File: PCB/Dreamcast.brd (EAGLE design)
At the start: 73 x 29 mm, 19 parts, among them U1 ESP32DEVKITC

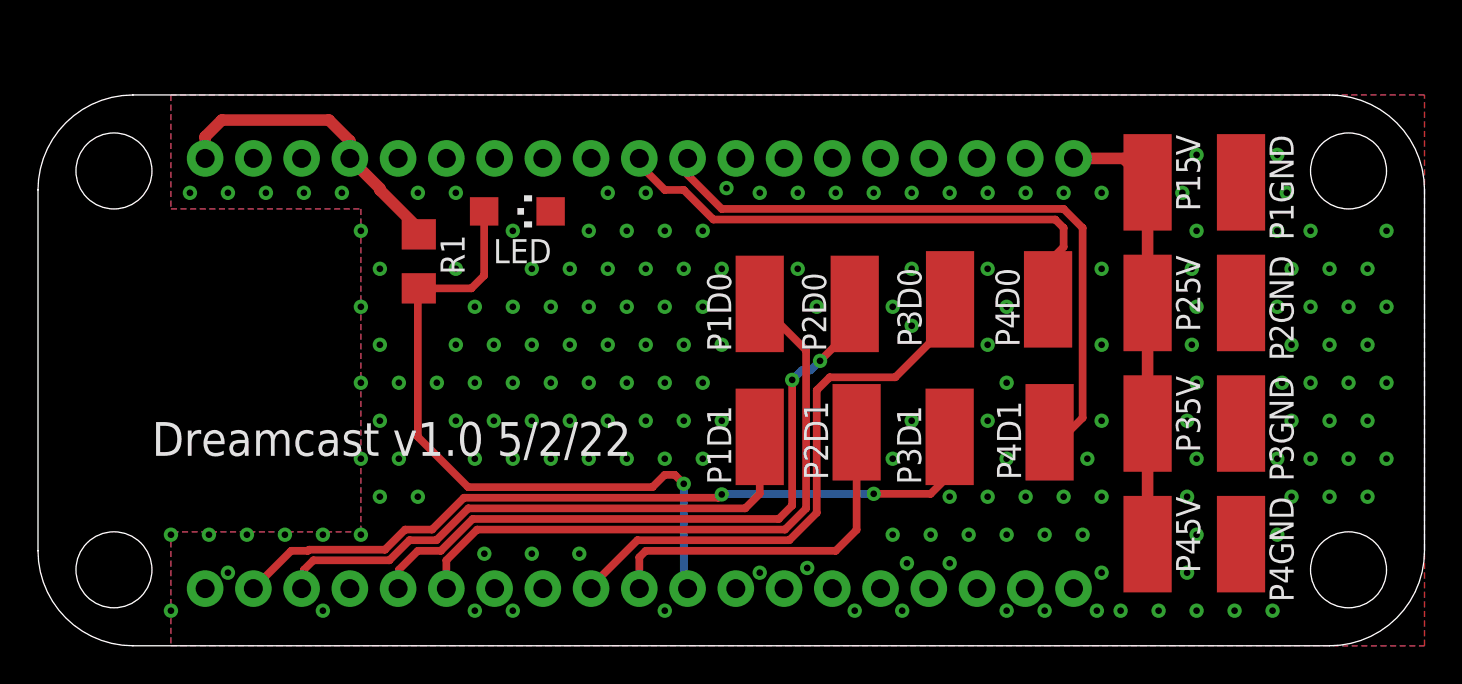
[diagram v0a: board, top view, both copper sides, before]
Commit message: Updated PCBs
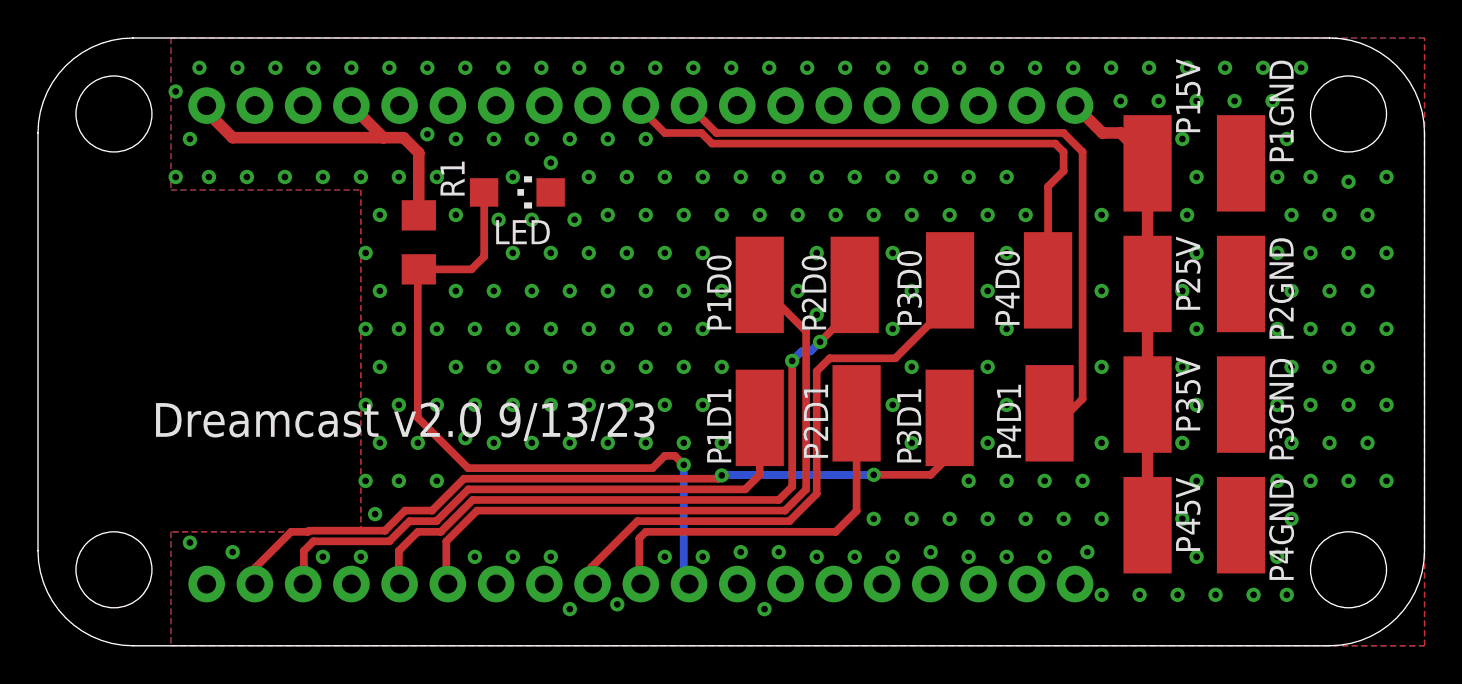
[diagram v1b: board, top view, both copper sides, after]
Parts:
- removed U1: ESP32DEVKITC, ESP32-DEVKITC:ESP32-DEVKITC
- added U2: ESP32DEVKITC, ESP32-DEVKITC4:ESP32-DEVKITC
- moved LED 1.00 mm to (25.2, 23.9)
- moved P15V 1.00 mm to (58.4, 25.4)
- moved P1D0 1.00 mm to (38.0, 19.0)
- moved P1D1 1.00 mm to (38.0, 12.0)
- moved P1GND 1.00 mm to (63.3, 25.4)
- moved P25V 1.00 mm to (58.4, 19.1)
- moved P2D0 1.00 mm to (43.0, 19.0)
- moved P2D1 1.00 mm to (43.1, 12.2)
- moved P2GND 1.00 mm to (63.3, 19.1)
- moved P35V 1.00 mm to (58.4, 12.7)
- moved P3D0 1.00 mm to (48.0, 19.2)
- moved P3D1 1.00 mm to (48.0, 12.0)
- moved P3GND 1.00 mm to (63.3, 12.7)
- moved P45V 1.00 mm to (58.4, 6.35)
- moved P4D0 1.00 mm to (53.2, 19.2)
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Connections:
- net 3V3: now also U2.1, U2.4; no longer U1.1, U1.4
- net 5V: now also U2.19; no longer U1.19
- net GND: now also U2.14, U2.31, U2.38, U2.5, U2.6, U2.7, U2.8, U2.9; no longer U1.14, U1.31, U1.38, U1.5, U1.6, U1.7, U1.8, U1.9
- net LED: now also U2.28; no longer U1.28
- net P1D0: now also U2.33; no longer U1.33
- net P1D1: now also U2.36; no longer U1.36
- net P2D0: now also U2.34; no longer U1.34
- net P2D1: now also U2.29; no longer U1.29
- net P3D0: now also U2.30; no longer U1.30
- net P3D1: now also U2.37; no longer U1.37
- net P4D0: now also U2.10; no longer U1.10
- net P4D1: now also U2.11; no longer U1.11
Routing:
- net P4D0: track 28.1 -> 30.5 mm
- net 3V3: track 16.0 -> 18.1 mm
- net P4D1: track 34.9 -> 36.8 mm
- net LED: track 36.1 -> 36.9 mm
- net P2D1: track 18.8 -> 19.6 mm
- net P3D0: track 29.8 -> 30.6 mm
- net P1D0: track 33.3 -> 34.1 mm
- net 5V: track 23.5 -> 24.2 mm
- net P2D0: track 35.4 -> 36.1 mm
- net P3D1: track 41.1 -> 41.9 mm
- net P1D1: track 29.7 -> 30.4 mm
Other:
- board size 73 x 29 mm -> 73 x 32 mm
- board text added: "Dreamcast v2.0 9/13/23"
- board text removed: "Dreamcast v1.0 5/2/22"
